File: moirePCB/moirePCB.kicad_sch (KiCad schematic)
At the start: 55 parts, among them J1 USB_C_Receptacle, U1 ESP32-PICO-D4, U1 TLC555xD, U10 TLV73333PDBV, U2 BQ25504, U3 TLV73333PDBV, U4 RFM95W-915S2, U5 CH340E, U7 HDC1080, U8 AP2281-1WG-7, U9 AP2281-1WG-7, Y2 32.768kHz

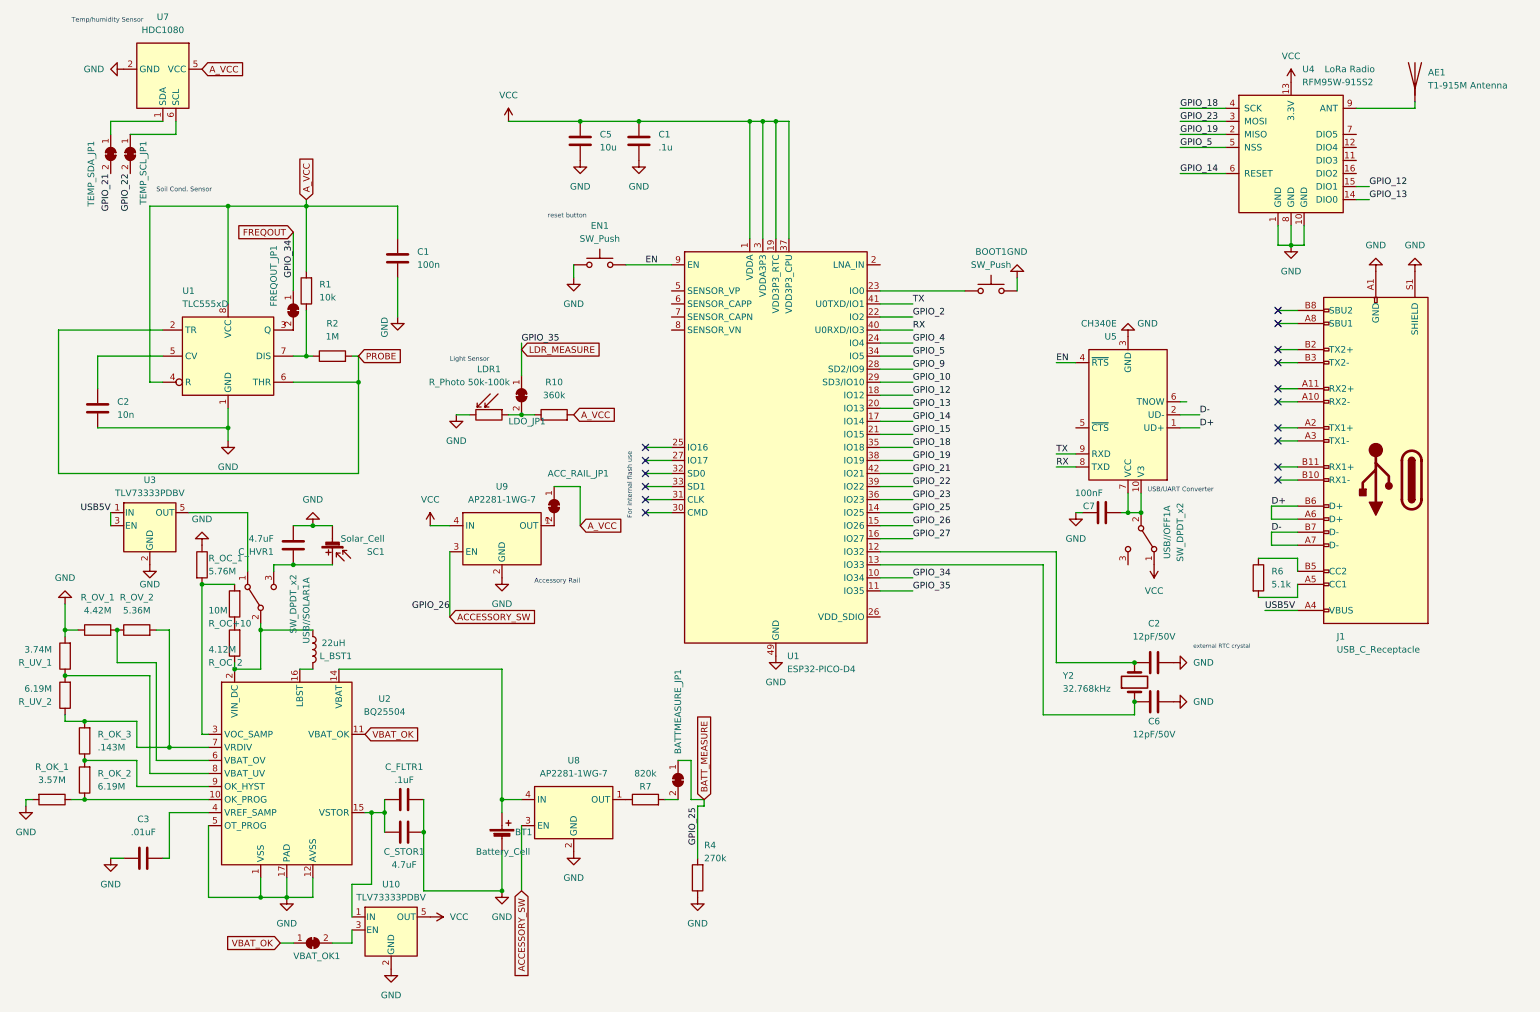
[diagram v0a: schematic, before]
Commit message: Daughter Board changes from meeting
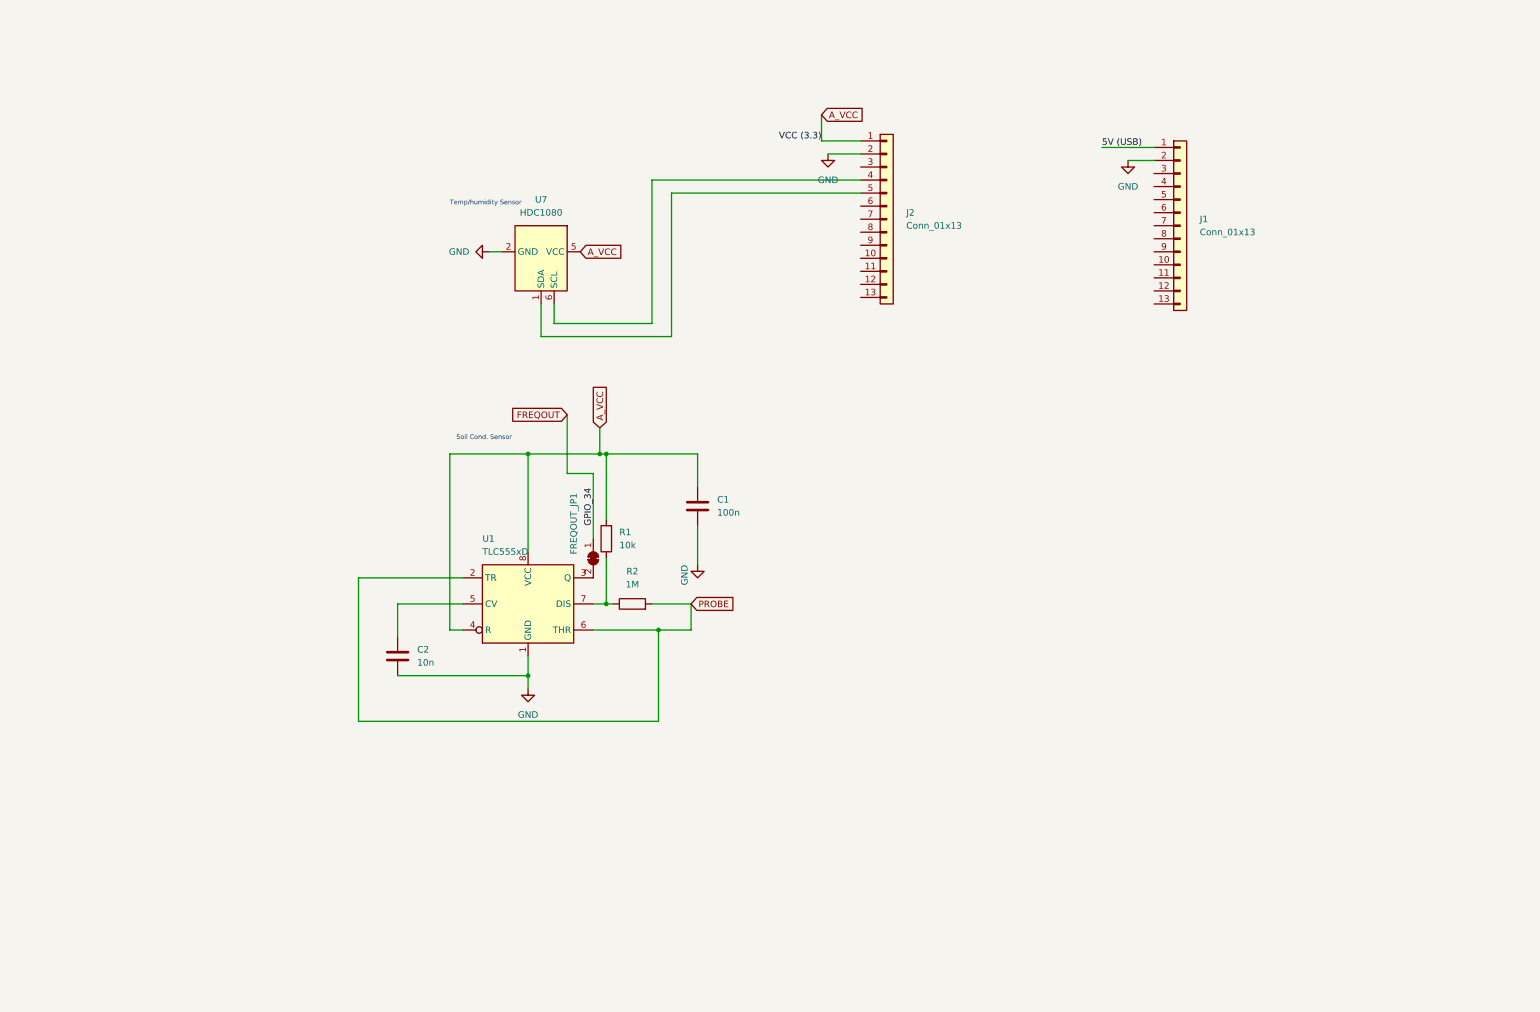
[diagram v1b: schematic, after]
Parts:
- removed ACC_RAIL_JP1, BATTMEASURE_JP1, LDO_JP1, TEMP_SCL_JP1, TEMP_SDA_JP1, VBAT_OK1: SolderJumper_2_Bridged, Jumper:SolderJumper-2_P1.3mm_Bridged_RoundedPad1.0x1.5mm, symbol Jumper:SolderJumper_2_Bridged
- removed AE1: T1-915M Antenna, Connector_PinHeader_2.54mm:PinHeader_1x01_P2.54mm_Vertical, symbol Device:Antenna
- removed BOOT1, EN1: SW_Push, Button_Switch_SMD:SW_Push_1P1T_XKB_TS-1187A, symbol Switch:SW_Push
- removed BT1: Battery_Cell, Connector_JST:JST_PH_S2B-PH-K_1x02_P2.00mm_Horizontal, symbol Device:Battery_Cell
- removed C1: .1u, Capacitor_SMD:C_0805_2012Metric, symbol Device:C
- removed C2, C6: 12pF/50V, Capacitor_SMD:C_0805_2012Metric, symbol Device:C
- removed C3: .01uF, Capacitor_SMD:C_0805_2012Metric, symbol Device:C
- removed C5: 10u, Capacitor_SMD:C_0805_2012Metric, symbol Device:C
- removed C7: 100nF, Capacitor_SMD:C_0805_2012Metric, symbol Device:C
- removed C_FLTR1: .1uF, Capacitor_SMD:C_0805_2012Metric, symbol Device:C
- removed C_HVR1, C_STOR1: 4.7uF, Capacitor_SMD:C_0805_2012Metric, symbol Device:C
- removed J1: USB_C_Receptacle, Connector_USB:USB_C_Receptacle_HRO_TYPE-C-31-M-12, symbol Connector:USB_C_Receptacle
- removed LDR1: R_Photo 50k-100k, Connector_PinHeader_2.54mm:PinHeader_1x02_P2.54mm_Horizontal, symbol Device:R_Photo
- removed L_BST1: 22uH, Inductor_SMD:L_0805_2012Metric, symbol Device:L
- removed R10: 360k, Resistor_SMD:R_0805_2012Metric, symbol Device:R
- removed R4: 270k, Resistor_SMD:R_0805_2012Metric, symbol Device:R
- removed R6: 5.1k, Resistor_SMD:R_0805_2012Metric, symbol Device:R
- removed R7: 820k, Resistor_SMD:R_0805_2012Metric, symbol Device:R
- removed R_OC+10: 10M, Resistor_SMD:R_0805_2012Metric, symbol Device:R
- removed R_OC_1: 5.76M, Resistor_SMD:R_0805_2012Metric, symbol Device:R
- removed R_OC_2: 4.12M, Resistor_SMD:R_0805_2012Metric, symbol Device:R
- removed R_OK_1: 3.57M, Resistor_SMD:R_0805_2012Metric, symbol Device:R
- removed R_OK_2, R_UV_2: 6.19M, Resistor_SMD:R_0805_2012Metric, symbol Device:R
- removed R_OK_3: .143M, Resistor_SMD:R_0805_2012Metric, symbol Device:R
- removed R_OV_1: 4.42M, Resistor_SMD:R_0805_2012Metric, symbol Device:R
- removed R_OV_2: 5.36M, Resistor_SMD:R_0805_2012Metric, symbol Device:R
- removed R_UV_1: 3.74M, Resistor_SMD:R_0805_2012Metric, symbol Device:R
- removed SC1: Solar_Cell, Connector_PinHeader_2.54mm:PinHeader_1x02_P2.54mm_Horizontal, symbol Device:Solar_Cell
- removed U1: ESP32-PICO-D4, Package_DFN_QFN:QFN-48-1EP_7x7mm_P0.5mm_EP5.3x5.3mm, symbol RF_Module:ESP32-PICO-D4
- removed U10, U3: TLV73333PDBV, Package_TO_SOT_SMD:SOT-23-5, symbol Regulator_Linear:TLV73333PDBV
- removed U2: BQ25504, Package_DFN_QFN:VQFN-16-1EP_3x3mm_P0.5mm_EP1.68x1.68mm, symbol Battery_Management:BQ25504
- removed U4: RFM95W-915S2, RF_Module:HOPERF_RFM9XW_SMD, symbol RF_Module:RFM95W-915S2
- removed U5: CH340E, Package_SO:MSOP-10_3x3mm_P0.5mm, symbol Interface_USB:CH340E
- removed U8, U9: AP2281-1WG-7, Package_TO_SOT_SMD:SOT-23-6, symbol Power_Management:AP2281-1WG-7
- removed USB//OFF1, USB//SOLAR1: SW_DPDT_x2, Button_Switch_SMD:SW_SPDT_PCM12, symbol Switch:SW_DPDT_x2
- removed Y2: 32.768kHz, Crystal:Crystal_SMD_MicroCrystal_CM9V-T1A-2Pin_1.6x1.0mm, symbol Device:Crystal
- added J1, J2: Conn_01x13, Connector_PinHeader_2.54mm:PinHeader_1x13_P2.54mm_Vertical, symbol Connector_Generic:Conn_01x13
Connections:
- net A_VCC: now also J2.1 (Pin_1)
- net GND: now also J1.2 (Pin_2), J2.2 (Pin_2)
- net at U7.1 (SDA): now also J2.5 (Pin_5)
- net at U7.6 (SCL): now also J2.4 (Pin_4)
- new net 5V (USB): J1.1 (Pin_1)
- no-connect marks 16 -> 0
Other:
- note removed: "Accessory Rail"
- note removed: "For internal flash use"
- note removed: "Light Sensor"
- note removed: "USB/UART Converter"
- note removed: "external RTC crystal"
- note removed: "reset button"
- moved on the sheet: C1, C2, FREQOUT_JP1, R1, R2, U1, U7
